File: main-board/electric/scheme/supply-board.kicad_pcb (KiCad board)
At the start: 2 copper layers, 74 x 56 mm, 136 parts, among them K1 CONN_3, P1 PWR-IN, P10 TST, P11 TST, P12 PWR-IN, P13 CONN_4, P14 PWR-IN, P16 TST, P2 PWR-IN, P3 CONN_4, P4 cross board conn, P5 PWR-IN, P6 TST, P7 TST, P8 TST, P9 CONN_3X2, Q1 BC847, Q10 MOS_N, Q11 MOS_P, Q12 MOS_P, Q2 BC847, Q3 BC847, Q4 MOS_P, Q5 BC847, Q6 BC857, Q7 BC847, Q8 BC857, Q9 BC847, U1 NCP3063, U2 L293, U3 MINI-USB-B, X1 8MHz

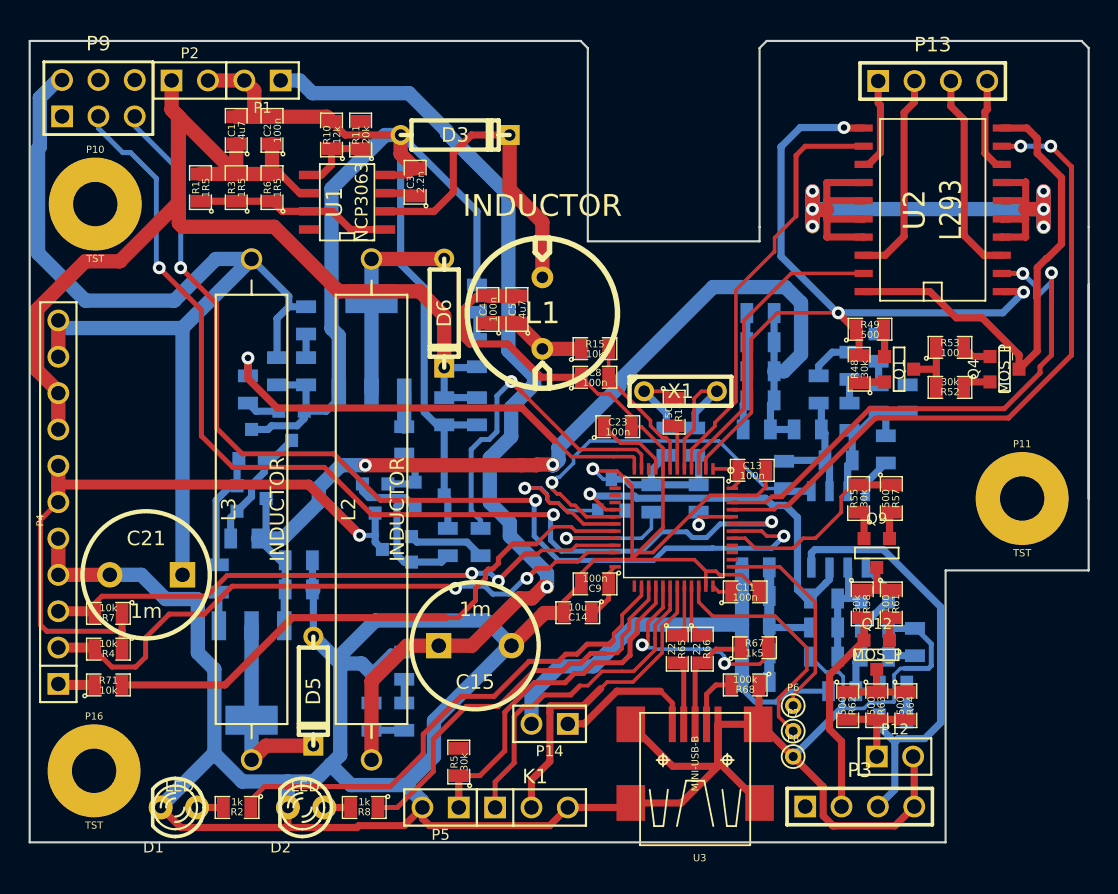
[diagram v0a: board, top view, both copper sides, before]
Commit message: Routing...
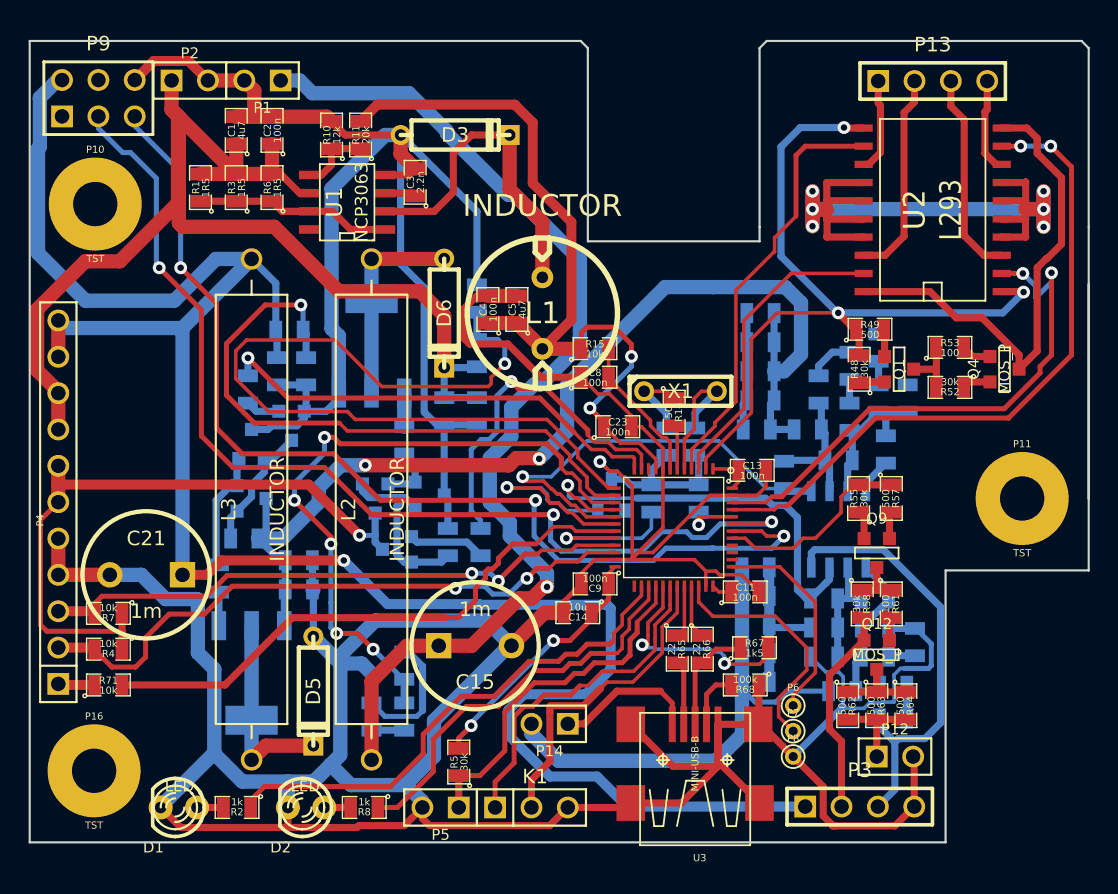
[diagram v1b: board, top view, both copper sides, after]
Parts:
- moved R46 1.37 mm to (161.7, 145.2), turned to 0 degrees
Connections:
- P9 pad 4: /buck-out-5v -> (no net)
- stm1 pad 13: /solar-volt -> /batt-volt
- stm1 pad 14: /batt-volt -> /buck-volt
- stm1 pad 15: /buck-volt -> /solar-volt
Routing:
- net /buck-out-5v: track 75.5 -> 142.5 mm, vias 0 -> 1
- net VDD: track 98.4 -> 155.8 mm, vias 1 -> 5
- net /batt-volt: track 1.91 -> 58.6 mm, vias 0 -> 1
- net /solar-volt: track 1.65 -> 51.2 mm, vias 0 -> 5
- net /buck-volt: track 1.65 -> 44.4 mm, vias 0 -> 1
- net GND: track 471.2 -> 483.0 mm
- net /boost-current: track 26.3 -> 30.6 mm
- net /buck-current: track 26.7 -> 30.3 mm
- net /solar: track 75.2 -> 78.4 mm
- net /temperature: track 13.5 -> 16.1 mm
- net /solar+: track 34.0 -> 35.9 mm
- net /buck+: track 73.2 -> 74.2 mm
- net /buck-pwm: track 32.8 -> 31.9 mm
